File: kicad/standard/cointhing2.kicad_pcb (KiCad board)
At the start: 2 copper layers, 35 x 34 mm, 29 parts, among them J1 USB_B_Micro, Q1 BC847BS, Q2 S8050_J3Y, U1 CP2102-GMR_NRND, U2 ESP-12E, U3 AMS1117-3.3

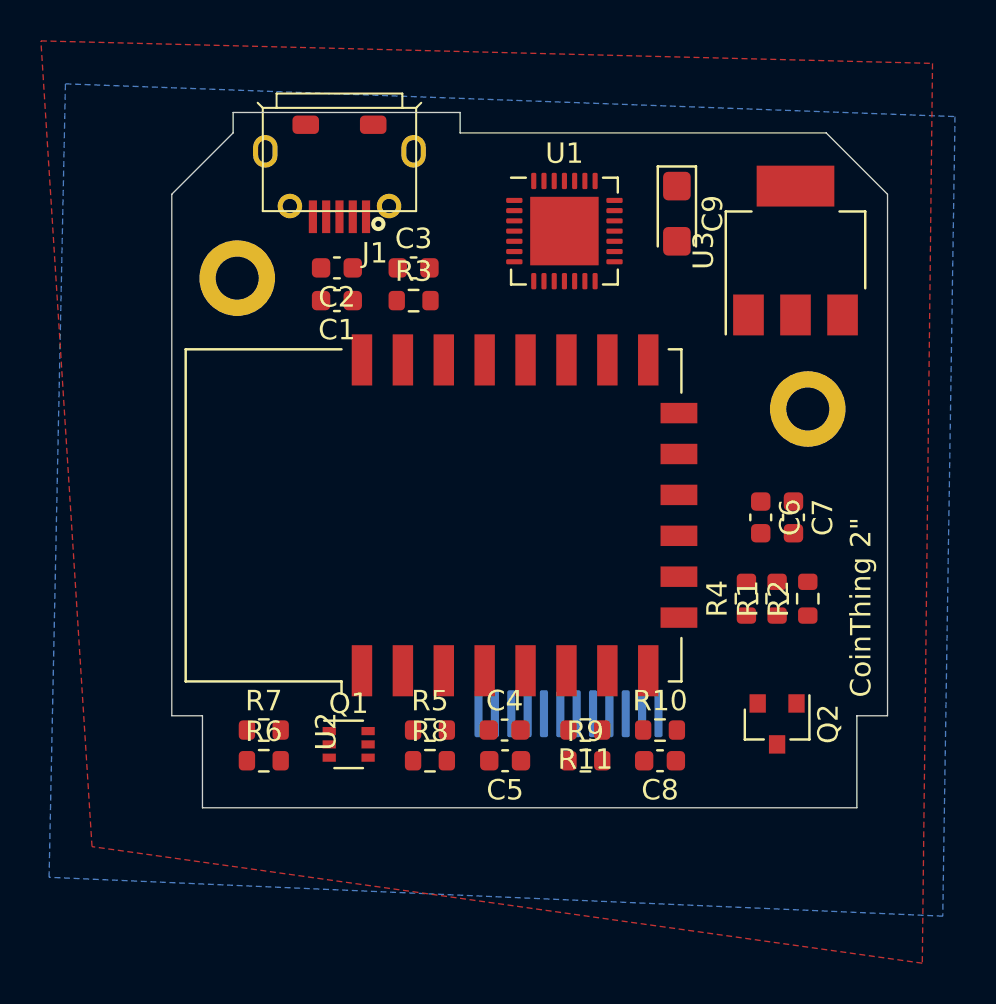
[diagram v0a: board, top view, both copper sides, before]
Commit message: Update cointhing2.kicad_pcb
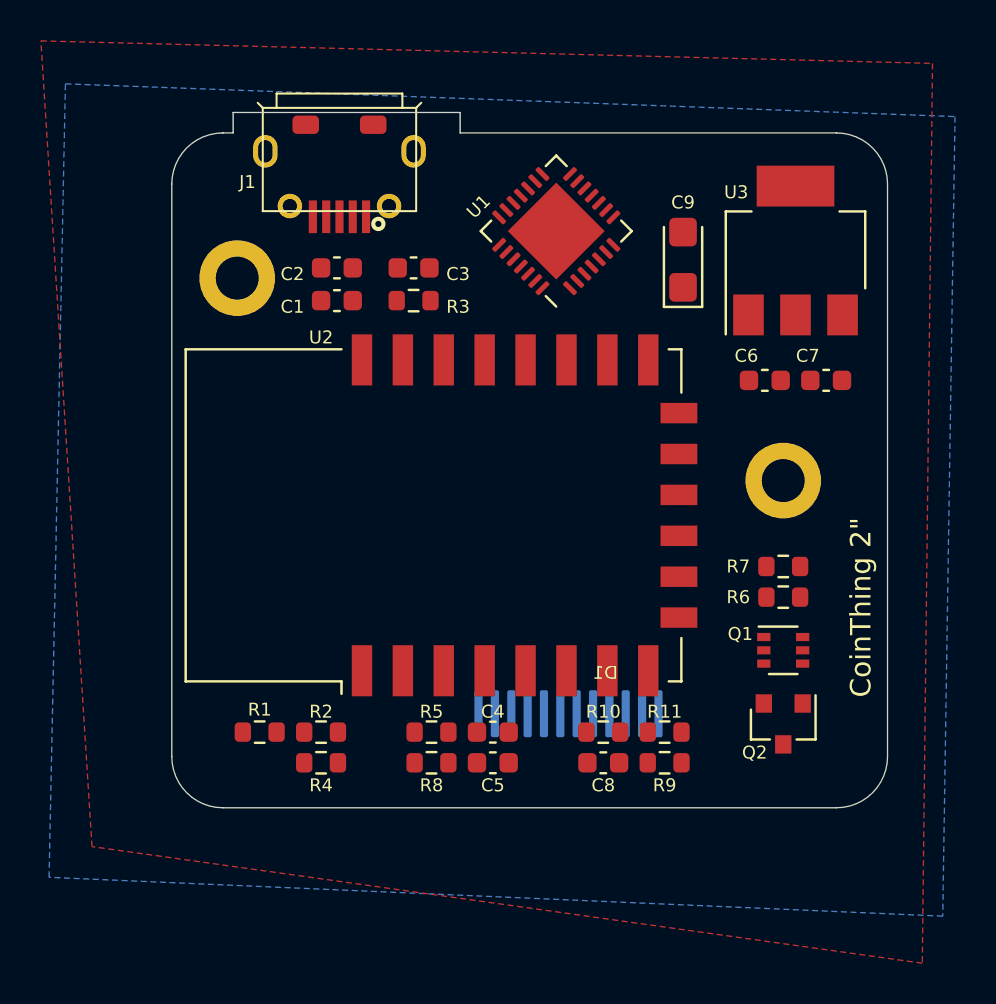
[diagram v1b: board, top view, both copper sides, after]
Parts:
- added QR*****: https://github.com/barn53/CoinThing/tree/2inch, https://github.com/barn53/CoinThing/tree/2inch, B.Cu at (170.8, 63.0)
- moved R6 26.6 mm to (174.9, 78.7)
- moved R7 26.6 mm to (174.9, 77.2)
- moved R1 26.1 mm to (149.3, 85.3), turned to 180 degrees
- moved R2 24.7 mm to (152.3, 85.3), turned to 180 degrees
- moved R4 22.3 mm to (152.3, 86.8), turned to 180 degrees
- moved Q1 21.7 mm to (174.9, 81.3)
- moved C7 6.89 mm to (177.0, 68.1), turned to 0 degrees
- moved C6 6.70 mm to (174.0, 68.1), turned to 180 degrees
- moved R11 3.88 mm to (169.1, 85.3), turned to 0 degrees
- moved R9 3.88 mm to (169.1, 86.8)
- moved REF** 3.70 mm to (171.4, 72.2)
- moved C8 2.78 mm to (166.1, 86.8)
- moved R10 2.78 mm to (166.1, 85.3), turned to 180 degrees
- moved C9 2.27 mm to (170.0, 62.2), turned to 90 degrees
- moved C5 0.61 mm to (160.7, 86.8)
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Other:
- outline, holes or cut-outs redrawn
